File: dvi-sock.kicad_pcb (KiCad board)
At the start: 2 copper layers, 25.2 x 22.5 mm, 14 parts, among them J1 Conn_01x05, J2 Conn_01x05, J3 Conn_01x03, J4 NOT_HDMI_A

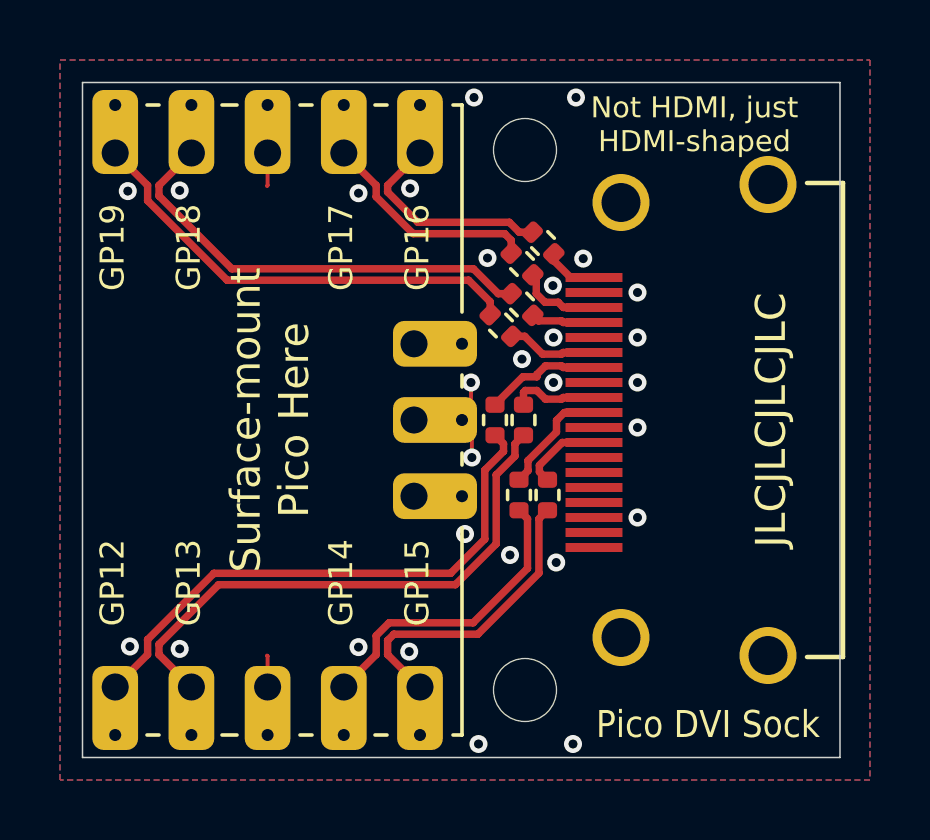
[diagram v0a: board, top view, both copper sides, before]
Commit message: Rounded corners, license, readme
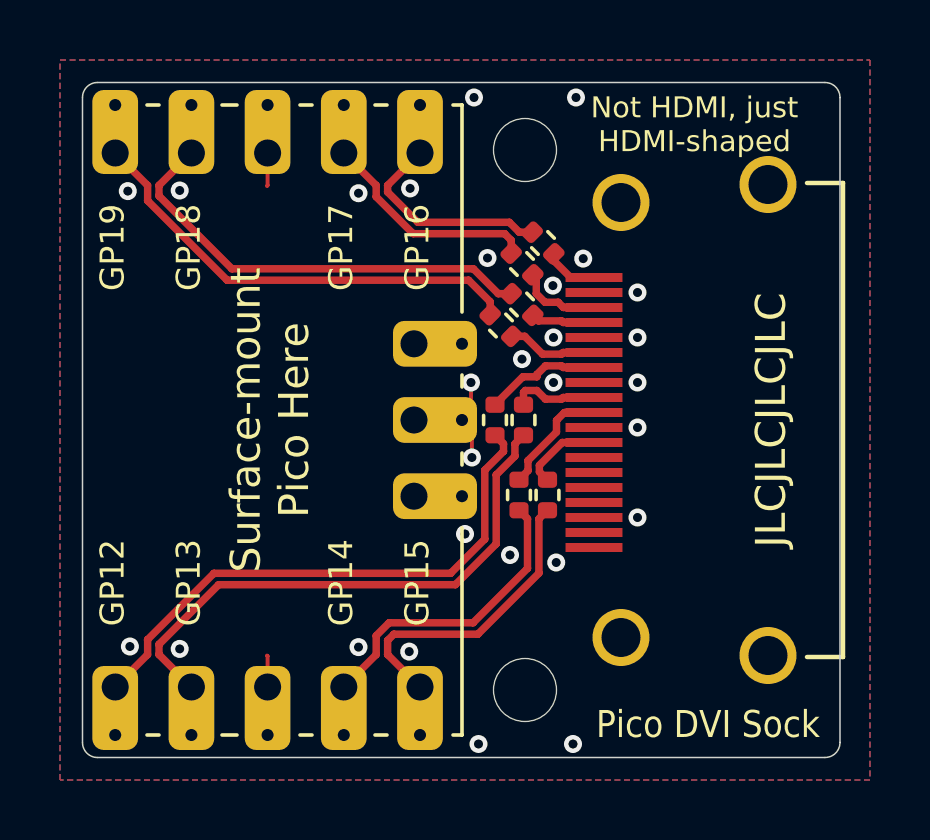
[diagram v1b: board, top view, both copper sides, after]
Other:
- outline, holes or cut-outs redrawn
- board text added: "Rev A"
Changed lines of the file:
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@@
   (gr_line (start 154.4 95.5) (end 154.1 95.5) (layer "F.SilkS") (width 0.12))
   (gr_line (start 146.4 95.5) (end 146.9 95.5) (layer "F.SilkS") (width 0.12))
-  (gr_line (start 167 96.25) (end 141.75 96.25) (layer "Edge.Cuts") (width 0.05))
-  (gr_line (start 141.75 73.75) (end 167 73.75) (layer "Edge.Cuts") (width 0.05))
-  (gr_line (start 141.75 96.25) (end 141.75 73.75) (layer "Edge.Cuts") (width 0.05))
-  (gr_line (start 167 73.75) (end 167 96.25) (layer "Edge.Cuts") (width 0.05))
+  (gr_arc (start 142.25 95.75) (end 142.25 96.25) (angle 90) (layer "Edge.Cuts") (width 0.05))
+  (gr_line (start 166.5 96.25) (end 142.25 96.25) (layer "Edge.Cuts") (width 0.05))
+  (gr_line (start 142.25 73.75) (end 166.5 73.75) (layer "Edge.Cuts") (width 0.05))
+  (gr_arc (start 166.5 74.25) (end 166.5 73.75) (angle 90) (layer "Edge.Cuts") (width 0.05))
+  (gr_arc (start 166.5 95.75) (end 167 95.75) (angle 90) (layer "Edge.Cuts") (width 0.05))
+  (gr_line (start 141.75 95.75) (end 141.75 74.25) (layer "Edge.Cuts") (width 0.05))
+  (gr_line (start 167 74.25) (end 167 95.75) (layer "Edge.Cuts") (width 0.05))
+  (gr_arc (start 142.25 74.25) (end 142.25 73.75) (angle -90) (layer "Edge.Cuts") (width 0.05))
   (gr_text "NOT HDMI" (at 163 85 90) (layer "B.SilkS")
     (effects (font (size 1 1) (thickness 0.25)) (justify mirror))
@@
     (effects (font (size 1 1) (thickness 0.15)) (justify mirror))
   )
+  (gr_text "Rev A" (at 162.25 95) (layer "B.SilkS")
+    (effects (font (size 0.7 0.7) (thickness 0.12)) (justify mirror))
+  )
   (gr_text "Pico DVI Sock" (at 162.6 95.15) (layer "F.SilkS")
